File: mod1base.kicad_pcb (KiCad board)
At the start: 2 copper layers, 100 x 100 mm, 171 parts, among them J1 COM, J10 12V 300mA, J11 FAN, J12 PWRSENSE, J2 SWD, J3 OUT, J4 IN, J5 LCD, J6 5034801000, J7 5034801000, J8 COM, J9 USB, Q1 IRLML6402, SW1 SOFT1, SW10 EVE-JBBF2020B, SW2 PRESETS, SW3 SOFT2, SW4 SOFT2, SW5 SOFT3, SW6 ALL_LOAD, SW7 STORE, SW8 STORE, SW9 EVE-JBBF2020B, U1 ATSAMD20G18A-AU, U2 LM1117DT-3.3, U3 74HCT245PW, U4 FT230XS, U5 AP3211

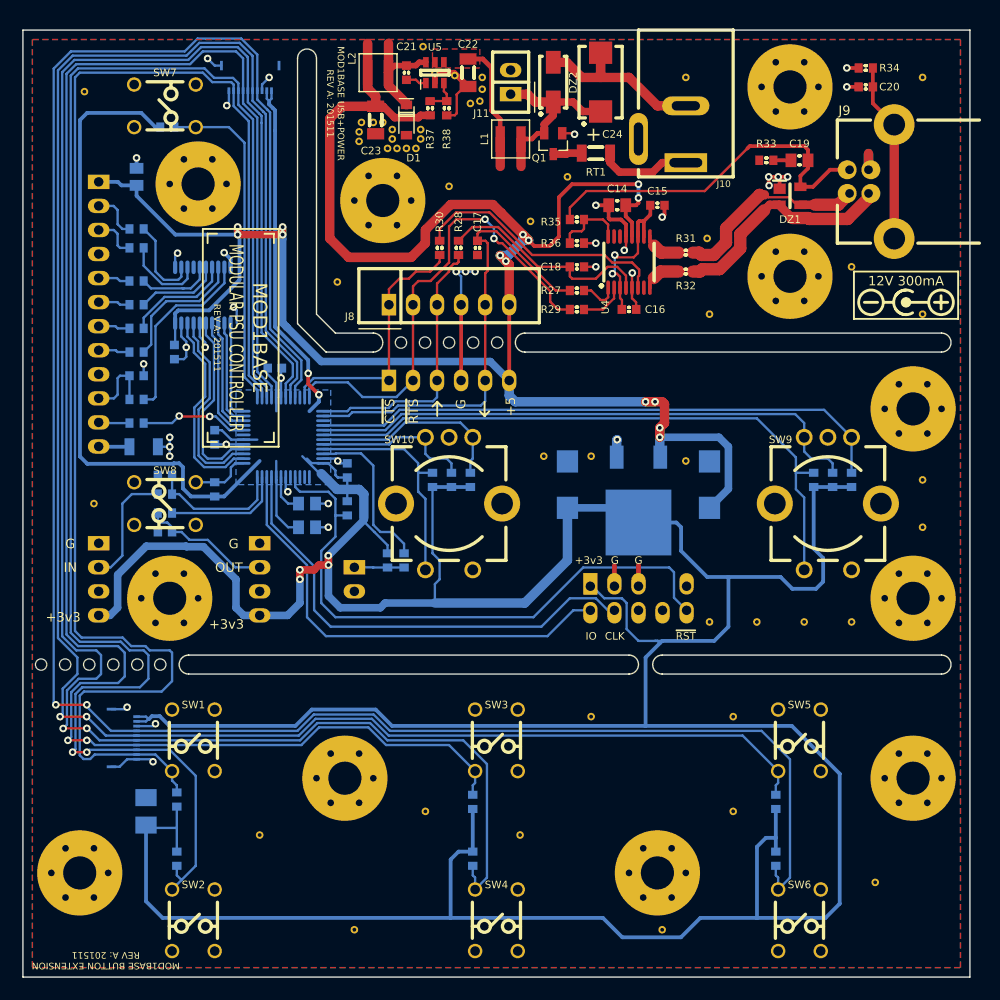
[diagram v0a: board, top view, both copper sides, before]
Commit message: More layout work
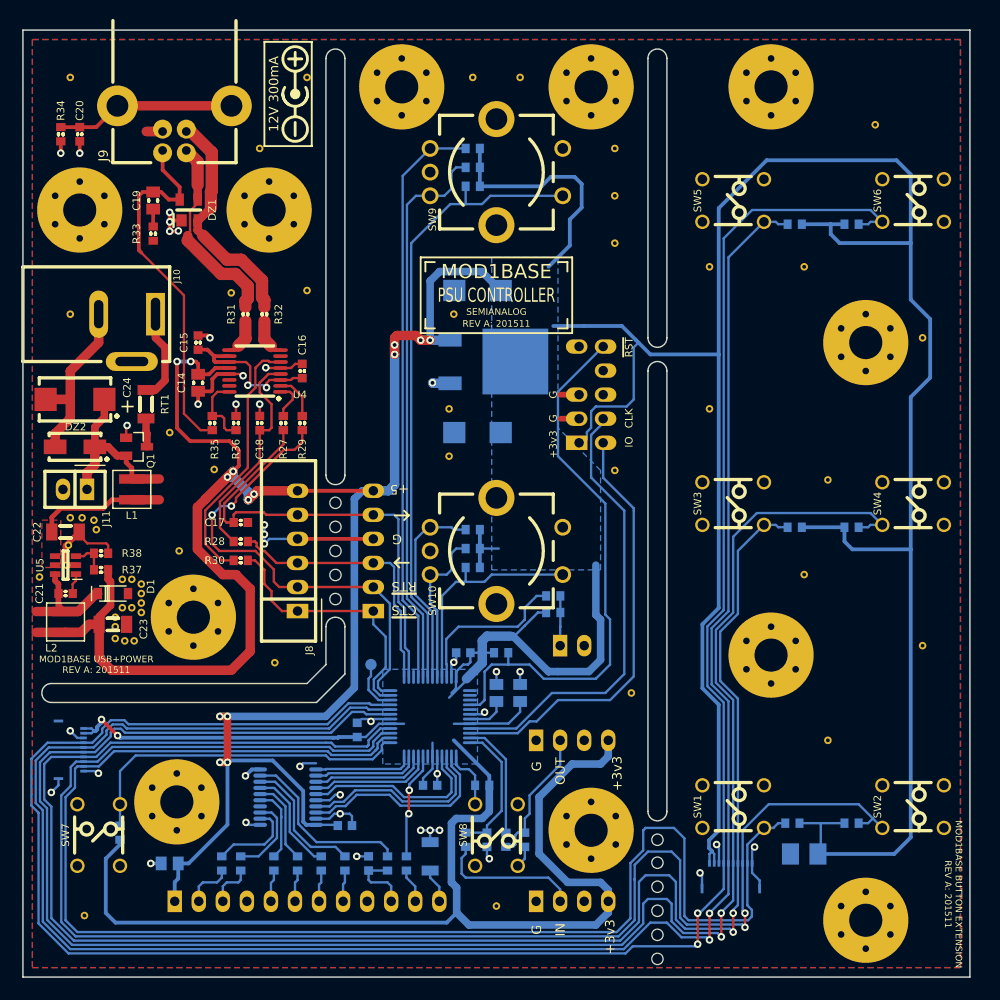
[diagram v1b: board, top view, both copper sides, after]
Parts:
- removed the REF** at (87.5, 62.5)
- removed the REF** at (72.5, 62.5)
- added REF**: VIA, VIA, F.Cu at (64.2, 70.0)
- added REF**: VIA, VIA, F.Cu at (62.5, 46.5)
- added REF**: VIA, VIA, F.Cu at (62.5, 12.5)
- added TP1: EXTRA, conn-test:TEST-SMD-SMALL, B.Cu at (36.8, 67.0)
- moved REF** 90.0 mm to (5.00, 5.00), turned to 90 degrees
- moved REF** 87.0 mm to (6.50, 93.5), turned to 90 degrees
- moved R34 85.3 mm to (4.00, 11.0), turned to 270 degrees
- moved C20 83.2 mm to (6.00, 11.0), turned to 270 degrees
- moved MP5 83.2 mm to (89.0, 94.0), turned to 90 degrees
- moved REF** 80.0 mm to (90.0, 10.0), turned to 90 degrees
- moved SW7 77.3 mm to (8.00, 85.0), turned to 180 degrees
- moved SW2 76.9 mm to (94.0, 82.0), turned to 90 degrees
- moved SW6 76.9 mm to (94.0, 18.0), turned to 90 degrees
- moved J9 76.4 mm to (16.0, 8.00), turned to 180 degrees
- moved MP9 76.1 mm to (6.00, 19.0), turned to 90 degrees
- moved R22 74.7 mm to (10.2, 84.8), turned to 270 degrees
- moved MP8 74.5 mm to (79.0, 6.00), turned to 90 degrees
- moved J6 73.5 mm to (5.00, 76.0), turned to 90 degrees
- moved C11 72.6 mm to (15.5, 88.0), turned to 180 degrees
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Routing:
- net +3.3: track 543.3 -> 489.9 mm, vias 6 -> 2
- net Net-(TP1-Pad1): track 0.00 -> 5.53 mm
- net /~RST: track 63.5 -> 58.6 mm
- net GND: track 119.5 -> 122.8 mm, vias 38 -> 39
- net Net-(J4-Pad2): track 12.7 -> 15.4 mm
- net /SWDIO: track 48.4 -> 45.8 mm
- net /SWCLK: track 50.1 -> 47.6 mm
- net /SW1: track 154.4 -> 155.9 mm
- net /SW2: track 167.3 -> 168.6 mm
- net /SW3: track 185.7 -> 187.0 mm
- net +5: track 223.9 -> 225.0 mm
- net /Rear breakaway/~CTS: track 27.4 -> 28.3 mm
- net /SW4: track 198.5 -> 199.4 mm
- net /SW5: track 212.8 -> 213.6 mm
- net /SW6: track 227.5 -> 228.3 mm
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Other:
- outline, holes or cut-outs redrawn
- board text added: "PSU CONTROLLER"
- board text added: "SEMIANALOG"
- board text removed: "MODULAR PSU CONTROLLER"
